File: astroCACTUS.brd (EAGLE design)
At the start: 57.7 x 135.1 mm, 21 parts, among them U1 ATTINY85-20P

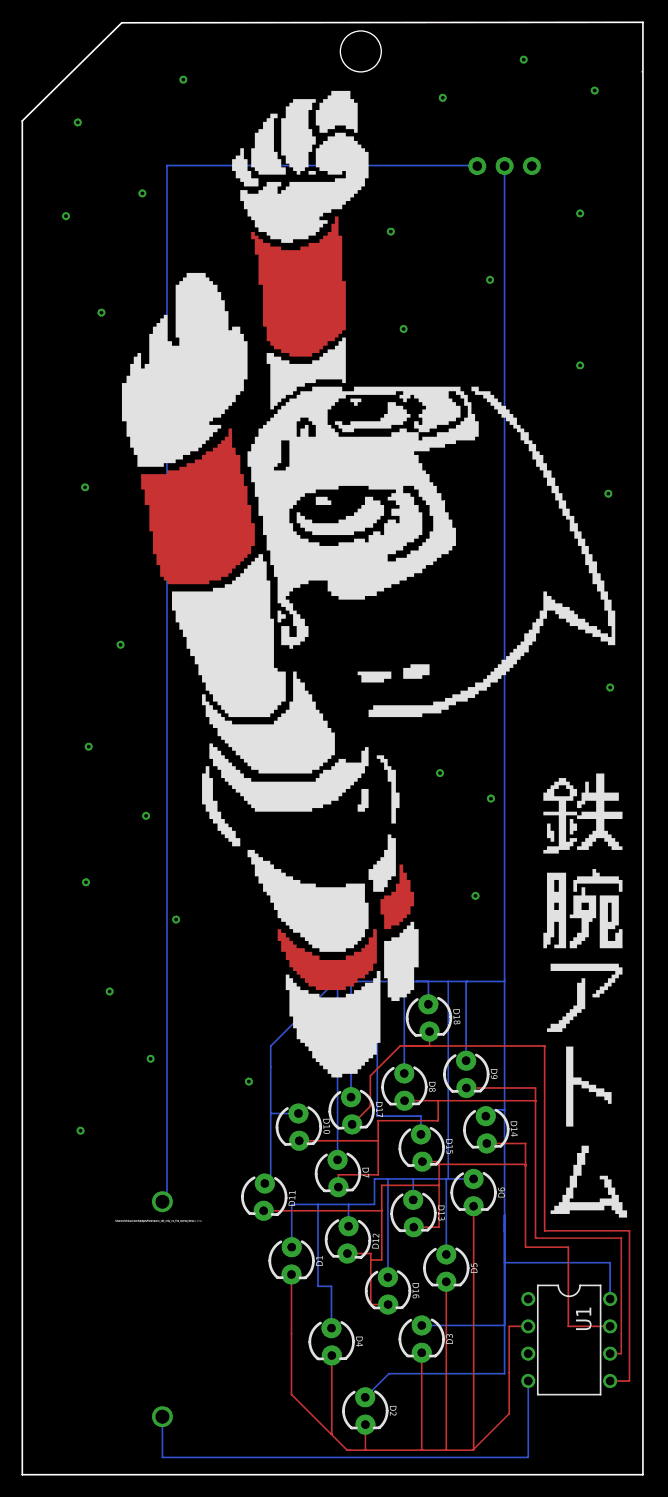
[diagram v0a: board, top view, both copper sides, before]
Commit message: astro boy
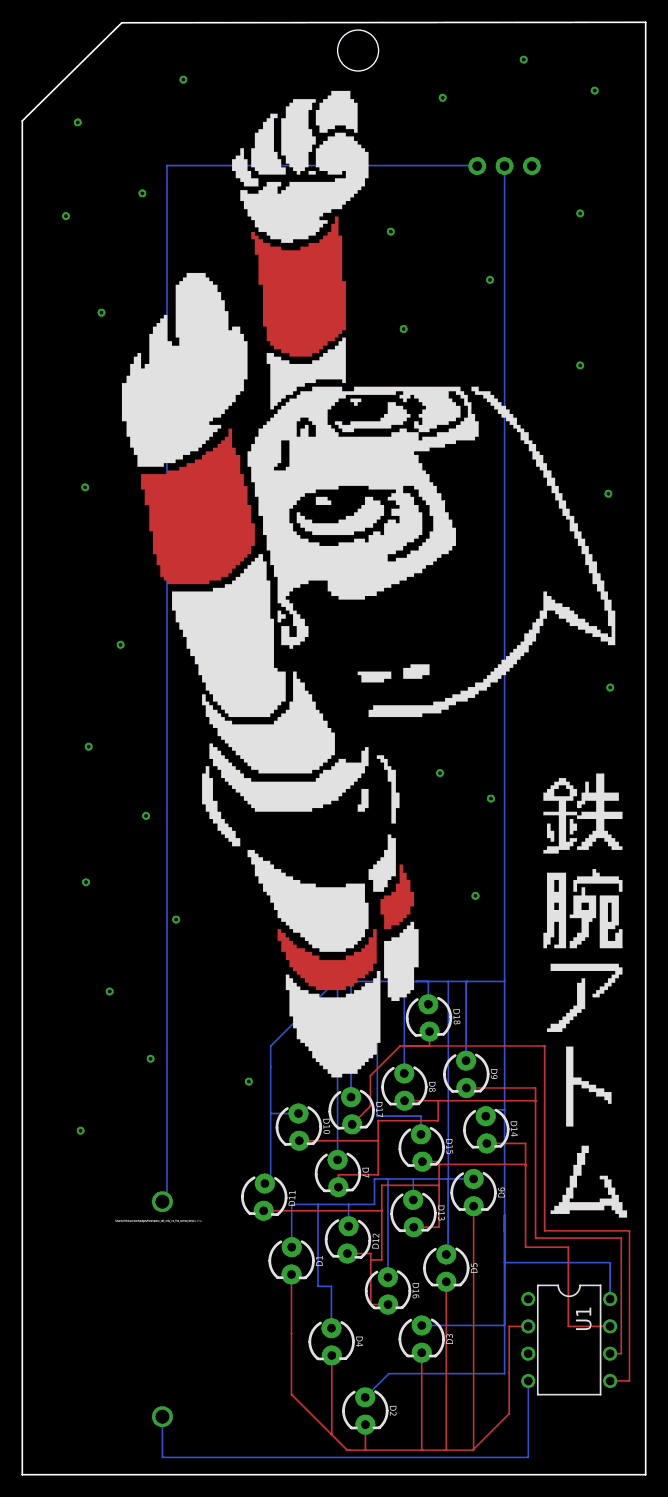
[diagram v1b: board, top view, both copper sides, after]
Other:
- board size 57.7 x 135.1 mm -> 58 x 135.1 mm
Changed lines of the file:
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@@
 <wire x1="-8.6351375" y1="-23.95826875" x2="-8.6351375" y2="101.985921875" width="0.1524" layer="20"/>
 <wire x1="-8.6351375" y1="101.985921875" x2="0.619725" y2="111.11258125" width="0.1524" layer="20"/>
-<wire x1="0.619725" y1="111.11258125" x2="49.101753125" y2="111.15621875" width="0.1524" layer="20"/>
-<wire x1="49.101753125" y1="111.15621875" x2="49.101753125" y2="-23.95826875" width="0.1524" layer="20"/>
-<wire x1="49.101753125" y1="-23.95826875" x2="-8.6351375" y2="-23.95826875" width="0.1524" layer="20"/>
-<rectangle x1="48.97881875" y1="106.46841875" x2="49.06518125" y2="106.553" layer="21"/>
-<rectangle x1="48.97881875" y1="106.553" x2="49.06518125" y2="106.63758125" layer="21"/>
+<wire x1="0.619725" y1="111.11258125" x2="49.355728125" y2="111.156221875" width="0.1524" layer="20"/>
+<wire x1="49.355728125" y1="111.156221875" x2="49.355728125" y2="-23.95826875" width="0.1524" layer="20"/>
+<wire x1="49.355728125" y1="-23.95826875" x2="-8.6351375" y2="-23.95826875" width="0.1524" layer="20"/>
 <rectangle x1="30.607" y1="66.59041875" x2="30.69081875" y2="66.675" layer="21"/>
 <rectangle x1="46.863" y1="-0.04241875" x2="47.625" y2="0.04241875" layer="21"/>
@@
 <rectangle x1="30.607" y1="66.59041875" x2="30.69081875" y2="66.675" layer="21"/>
 <text x="0" y="-0.42418125" size="0.17018125" layer="21" font="vector">/Users/chrisbuckner/badges/fresh/astro_silk_only_no_fire_words_bitmap.bmp</text>
-<hole x="22.8577125" y="108.44715625" drill="3.81"/>
+<hole x="22.6037375" y="108.5318125" drill="3.81"/>
 </plain>
 <attributes>
@@
 <wire x1="18.878778125" y1="1.10055625" x2="18.878778125" y2="1.185215625" width="0.1524" layer="16"/>
 <wire x1="20.12576875" y1="-6.434021875" x2="18.878778125" y2="-6.434021875" width="0.1524" layer="16"/>
-<wire x1="30.807715625" y1="-3.470478125" x2="30.807715625" y2="3.556153125" width="0.1524" layer="16"/>
-<wire x1="30.807715625" y1="3.556153125" x2="30.90024375" y2="3.556153125" width="0.1524" layer="16"/>
+<wire x1="30.97703125" y1="-3.3011625" x2="30.97703125" y2="3.556153125" width="0.1524" layer="16"/>
+<wire x1="30.90024375" y1="3.556153125" x2="30.97703125" y2="3.556153125" width="0.1524" layer="16"/>
 <wire x1="36.233709375" y1="0.169315625" x2="36.233709375" y2="9.98966875" width="0.1524" layer="16"/>
 <wire x1="25.46690625" y1="-14.56073125" x2="36.233709375" y2="-14.56073125" width="0.1524" layer="16"/>
@@
 <wire x1="36.23370625" y1="-0.676765625" x2="36.23370625" y2="-1.35453125" width="0.1524" layer="16"/>
 <wire x1="36.233709375" y1="-1.35453125" x2="36.23370625" y2="-1.35453125" width="0.1524" layer="16"/>
+<wire x1="30.807715625" y1="-3.470478125" x2="30.97703125" y2="-3.3011625" width="0.1524" layer="16"/>
 </signal>
 <signal name="N$1">
